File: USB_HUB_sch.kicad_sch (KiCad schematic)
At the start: 32 parts, among them IC1 USB2513B_M2, U10 TPD2EUSB30ADRTR, U11 TPD2EUSB30ADRTR, U12 TPD2EUSB30ADRTR, Y1 MURATA_XRCGB24M000FFS1DR0

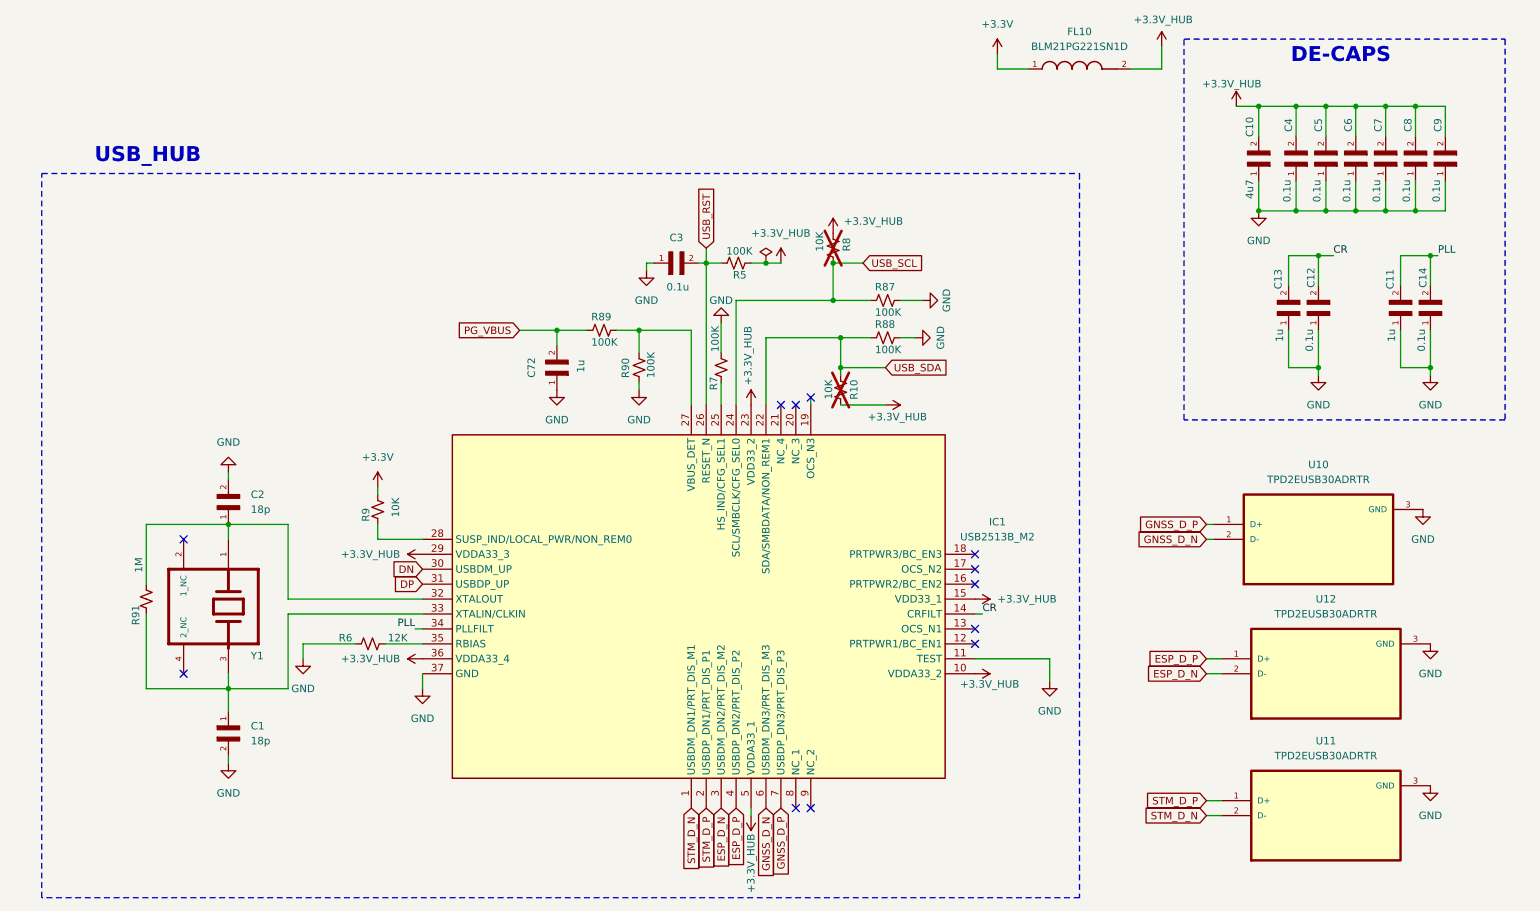
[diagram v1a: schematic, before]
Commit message: new
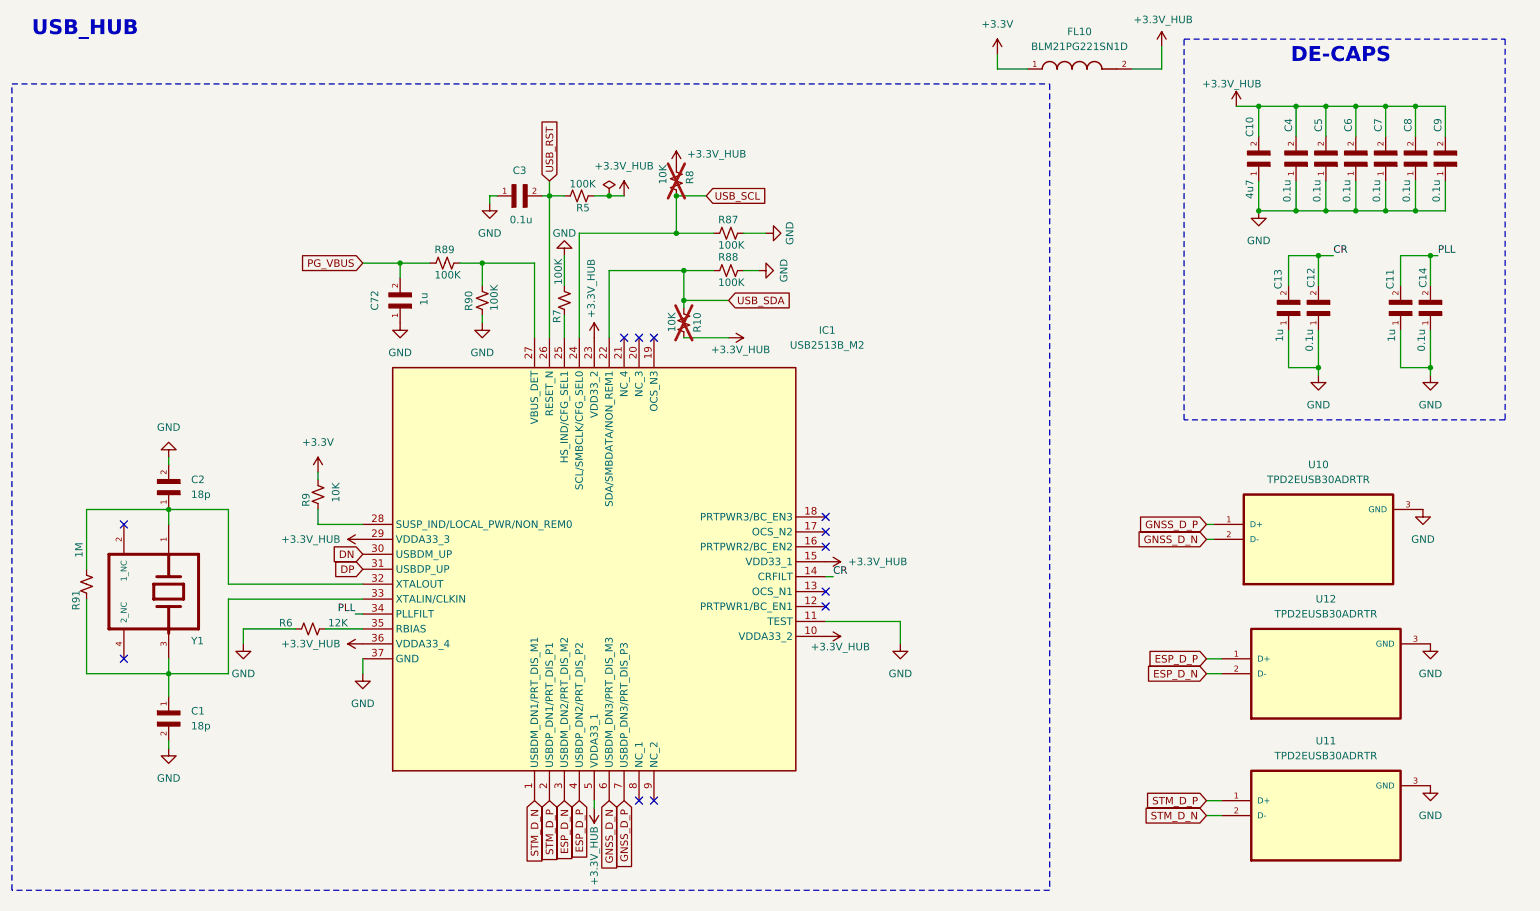
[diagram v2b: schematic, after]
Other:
- moved on the sheet: C1, C2, C3, C72, IC1, R10, R5, R6, R7, R8, R87, R88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

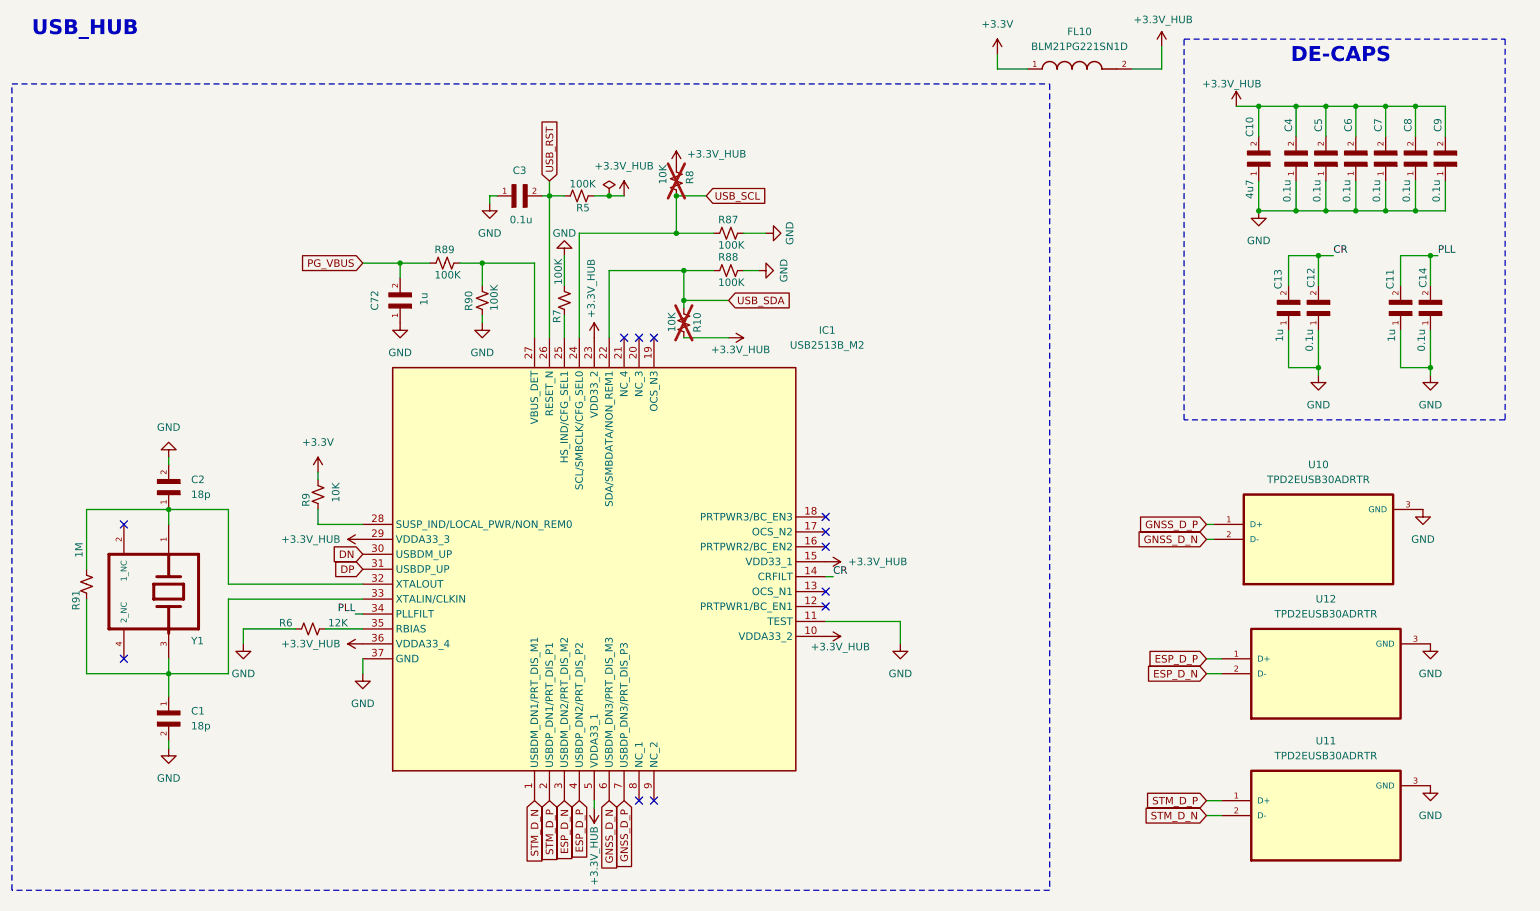
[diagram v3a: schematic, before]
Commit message: full
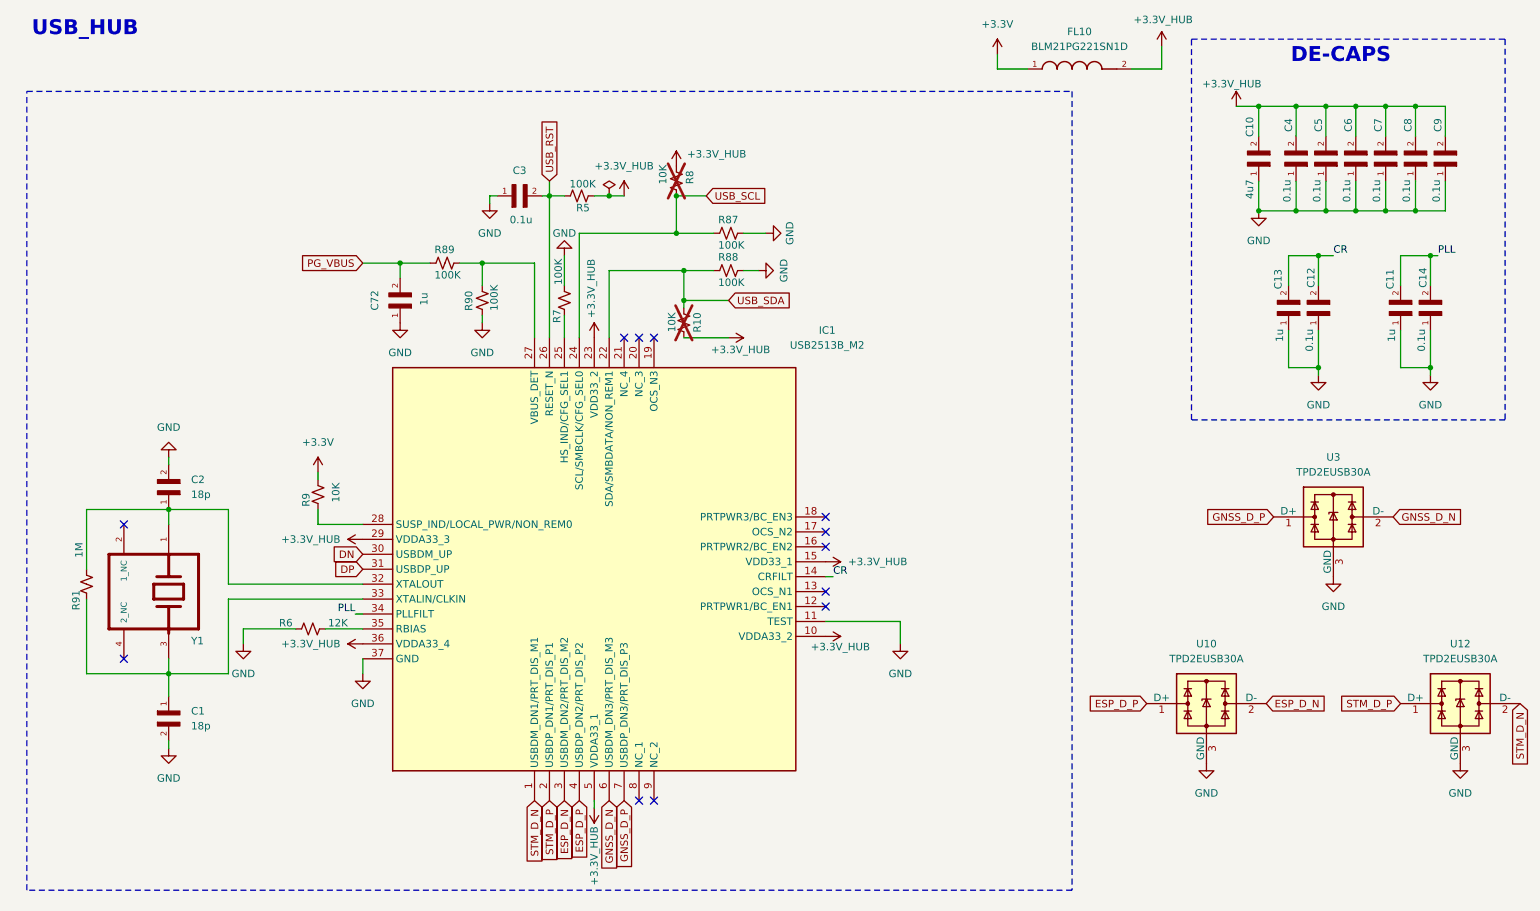
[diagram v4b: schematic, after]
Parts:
- removed U10, U11, U12: TPD2EUSB30ADRTR, GNSS:SOTFL35P100X50-3N, symbol TPD2EUSB30ADRTR:TPD2EUSB30ADRTR
- added U10, U12, U3: TPD2EUSB30A, Package_TO_SOT_SMD:Texas_DRT-3, symbol Power_Protection:TPD2EUSB30A
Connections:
- net ESP_D_N: now also U10.2 (D-)
- net ESP_D_P: now also U10.1 (D+)
- net GND: now also U10.3 (GND), U12.3 (GND), U3.3 (GND)
- net GNSS_D_N: now also U3.2 (D-)
- net GNSS_D_P: now also U3.1 (D+)
- net STM_D_N: now also U12.2 (D-)
- net STM_D_P: now also U12.1 (D+)
